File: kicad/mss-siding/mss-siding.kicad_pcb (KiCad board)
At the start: 2 copper layers, 82.6 x 76.2 mm, 108 parts, among them J1 Screw_Terminal_01x02, J10 Screw_Terminal_01x02, J11 Molex 0532610471, J12 Molex 0532610471, J2 SM04B-SRSS, J3 SM04B-SRSS, J4 SM04B-SRSS, J5 8P8C, J6 8P8C, J7 AVR-ISP, J8 Screw_Terminal_01x02, J9 Screw_Terminal_01x02, SW1 JS202011SCQN, U1 AP7381-50Y, U2 ATtiny861A-S, U3 74HC4049, U4 AP3012

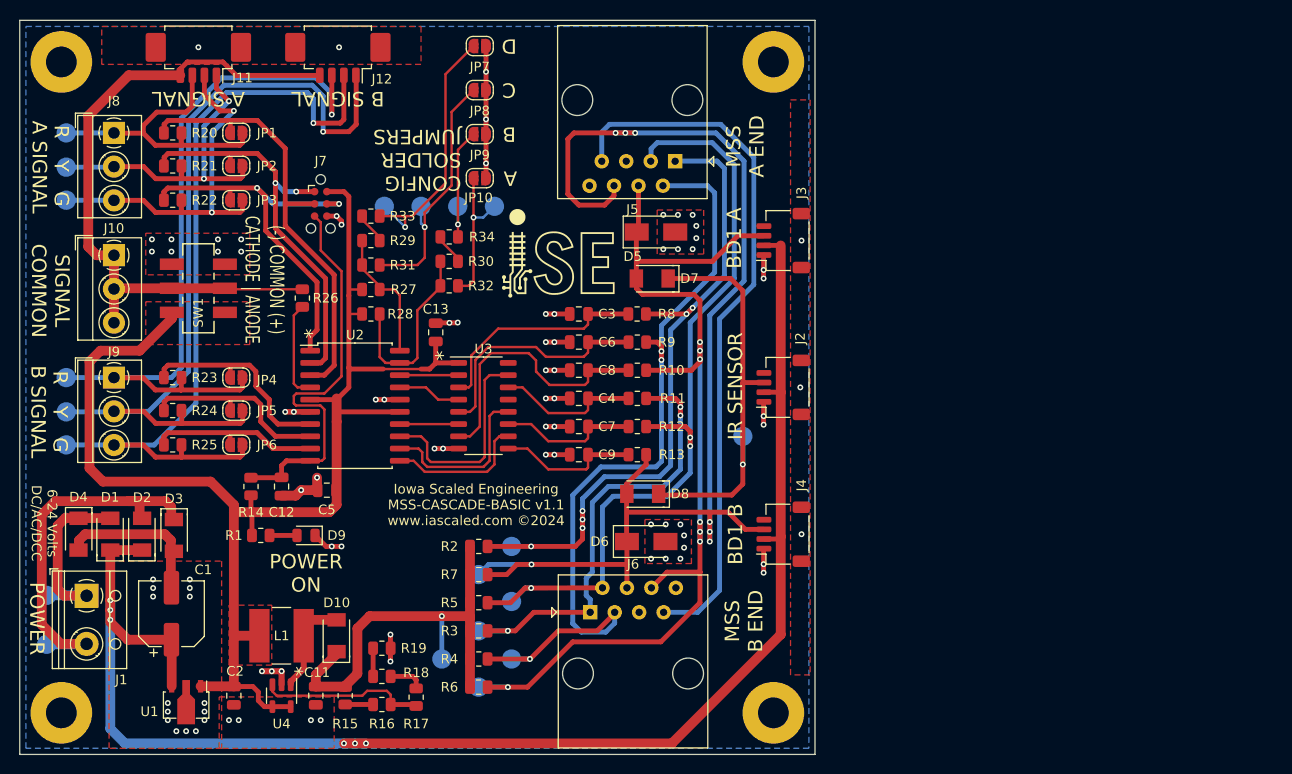
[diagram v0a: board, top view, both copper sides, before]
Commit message: First cut of PCB
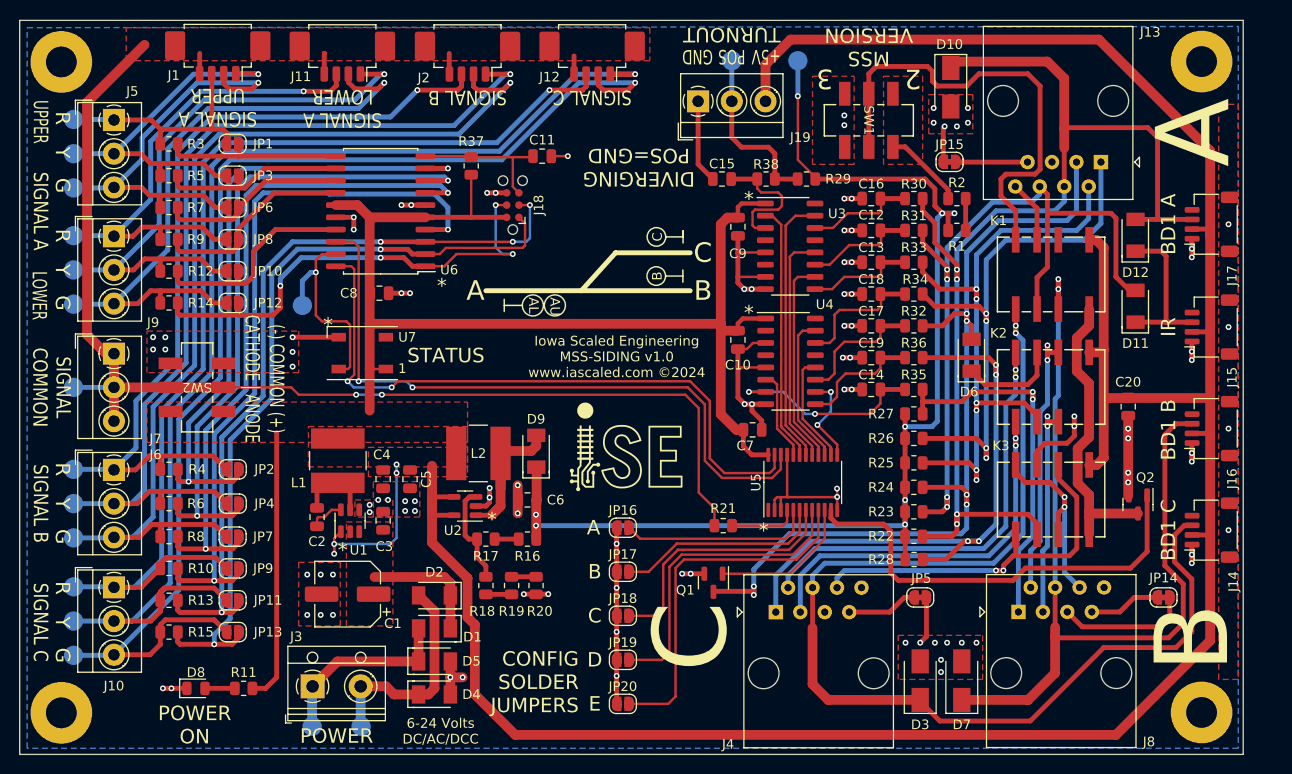
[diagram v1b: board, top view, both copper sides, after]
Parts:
- removed TP19, TP20: TestPoint, TestPoint:TestPoint_Pad_D2.0mm
- added C10: 0.1uF, Capacitor_SMD:C_0805_2012Metric, F.Cu at (99.9, 148.7)
- added C14: 0.1uF, Capacitor_SMD:C_0805_2012Metric, F.Cu at (113.8, 153.9)
- added C15: 0.1uF, Capacitor_SMD:C_0805_2012Metric, F.Cu at (98.3, 132.0)
- added C16: 0.1uF, Capacitor_SMD:C_0805_2012Metric, F.Cu at (113.8, 134.1)
- added C17: 0.1uF, Capacitor_SMD:C_0805_2012Metric, F.Cu at (113.8, 147.3)
- added C18: 0.1uF, Capacitor_SMD:C_0805_2012Metric, F.Cu at (113.8, 144.0)
- added C19: 0.1uF, Capacitor_SMD:C_0805_2012Metric, F.Cu at (113.8, 150.6)
- added C20: 10uF, Capacitor_SMD:C_0805_2012Metric, F.Cu at (140.5, 155.7)
- added D11: CDBM140G, ISE_Generic:SOD-123T, F.Cu at (141.2, 145.2)
- added D12: CDBM140G, ISE_Generic:SOD-123T, F.Cu at (141.2, 137.9)
- added J13: 8P8C, Connector_RJ:RJ45_Amphenol_54602-x08_Horizontal, F.Cu at (137.6, 130.3)
- added J14: SM04B-SRSS, Connector_JST:JST_SH_SM04B-SRSS-TB_1x04-1MP_P1.00mm_Horizontal, F.Cu at (149.1, 168.5)
- added J15: SM04B-SRSS, Connector_JST:JST_SH_SM04B-SRSS-TB_1x04-1MP_P1.00mm_Horizontal, F.Cu at (149.1, 147.4)
- added J16: SM04B-SRSS, Connector_JST:JST_SH_SM04B-SRSS-TB_1x04-1MP_P1.00mm_Horizontal, F.Cu at (149.1, 157.9)
- added J17: SM04B-SRSS, Connector_JST:JST_SH_SM04B-SRSS-TB_1x04-1MP_P1.00mm_Horizontal, F.Cu at (149.1, 136.7)
- added J18: AVR-ISP, Connector:Tag-Connect_TC2030-IDC-NL_2x03_P1.27mm_Vertical, F.Cu at (76.6, 134.7)
- added J19: Screw_Terminal_01x02, TerminalBlock_MetzConnect:TerminalBlock_MetzConnect_Type059_RT06303HBWC_1x03_P3.50mm_Horizontal, F.Cu at (95.8, 124.0)
- added JP11: SolderJumper_2_Open, Jumper:SolderJumper-2_P1.3mm_Open_RoundedPad1.0x1.5mm, F.Cu at (47.5, 175.8)
- added JP12: SolderJumper_2_Open, Jumper:SolderJumper-2_P1.3mm_Open_RoundedPad1.0x1.5mm, F.Cu at (47.5, 144.9)
- added JP13: SolderJumper_2_Open, Jumper:SolderJumper-2_P1.3mm_Open_RoundedPad1.0x1.5mm, F.Cu at (47.5, 179.1)
- added JP14: SolderJumper_2_Bridged, Jumper:SolderJumper-2_P1.3mm_Bridged_RoundedPad1.0x1.5mm, F.Cu at (144.1, 175.5)
- added JP15: SolderJumper_2_Bridged, Jumper:SolderJumper-2_P1.3mm_Bridged_RoundedPad1.0x1.5mm, F.Cu at (121.9, 130.3)
- added JP16: SolderJumper_2_Open, Jumper:SolderJumper-2_P1.3mm_Open_RoundedPad1.0x1.5mm, F.Cu at (88.0, 168.2)
- added JP17: SolderJumper_2_Open, Jumper:SolderJumper-2_P1.3mm_Open_RoundedPad1.0x1.5mm, F.Cu at (88.0, 172.8)
- added JP18: SolderJumper_2_Open, Jumper:SolderJumper-2_P1.3mm_Open_RoundedPad1.0x1.5mm, F.Cu at (88.0, 177.4)
- added JP19: SolderJumper_2_Open, Jumper:SolderJumper-2_P1.3mm_Open_RoundedPad1.0x1.5mm, F.Cu at (88.0, 182.0)
- added JP20: SolderJumper_2_Open, Jumper:SolderJumper-2_P1.3mm_Open_RoundedPad1.0x1.5mm, F.Cu at (88.0, 186.5)
- added K1: AGQ200A4H, ISE_UltraLibrarian:RELAY_AGQ_A_PAN, F.Cu at (132.5, 141.9)
- added K2: AGQ200A4H, ISE_UltraLibrarian:RELAY_AGQ_A_PAN, F.Cu at (132.5, 153.6)
- added K3: AGQ200A4H, ISE_UltraLibrarian:RELAY_AGQ_A_PAN, F.Cu at (132.5, 165.3)
- added L2: 4.7uH, ISE_UltraLibrarian:MSS6132-xxxMLC, F.Cu at (73.0, 160.5)
- added Q1: ZXMS6004FF, Package_TO_SOT_SMD:SOT-23, F.Cu at (97.4, 174.0)
- added Q2: DRDC3105-7, Package_TO_SOT_SMD:SOT-23, F.Cu at (141.5, 165.8)
- added R35: 10k, Resistor_SMD:R_0805_2012Metric, F.Cu at (118.2, 153.9)
- added R36: 10k, Resistor_SMD:R_0805_2012Metric, F.Cu at (118.2, 150.6)
- added R37: 10k, Resistor_SMD:R_0805_2012Metric, F.Cu at (72.3, 130.7)
- added R38: 10k, Resistor_SMD:R_0805_2012Metric, F.Cu at (102.9, 132.0)
- added SW2: JS202011SCQN, ISE_UltraLibrarian:SW_JS202011SCQN, F.Cu at (43.8, 153.7)
- added U5: PCA9555PW, Package_SO:TSSOP-24_4.4x7.8mm_P0.65mm, F.Cu at (106.7, 163.5)
- added U6: ATtiny861A-S, Package_SO:SOIC-20W_7.5x12.8mm_P1.27mm, F.Cu at (62.9, 135.4)
- added U7: WS2812B, LED_SMD:LED_WS2812B_PLCC4_5.0x5.0mm_P3.2mm, F.Cu at (61.0, 150.1)
- C11: value 10uF -> 1uF
- C12: value 1uF -> 0.1uF
- C2: value 22uF -> 0.1uF
- C3, C6: value 0.1uF -> 10uF
- C4, C5: value 0.1uF -> 22uF
- D10, D3, D7: value CDBM140G -> SMAJ18A-TP; footprint ISE_Generic:SOD-123T -> Diode_SMD:D_SMA
- D5, D6: value SMAJ18A-TP -> CDBM140G; footprint Diode_SMD:D_SMA -> ISE_Generic:SOD-123T
- D8: value CDBM140G -> GREEN LED; footprint ISE_Generic:SOD-123T -> LED_SMD:LED_0805_2012Metric
- D9: value GREEN LED -> CDBM140G; footprint LED_SMD:LED_0805_2012Metric -> ISE_Generic:SOD-123T
- J1: value Screw_Terminal_01x02 -> Molex 0532610471; footprint TerminalBlock_RND:TerminalBlock_RND_205-00012_1x02_P5.00mm_Horizontal -> Connector_Molex:Molex_PicoBlade_53261-0471_1x04-1MP_P1.25mm_Horizontal
- J2: value SM04B-SRSS -> Molex 0532610471; footprint Connector_JST:JST_SH_SM04B-SRSS-TB_1x04-1MP_P1.00mm_Horizontal -> Connector_Molex:Molex_PicoBlade_53261-0471_1x04-1MP_P1.25mm_Horizontal
- J3: value SM04B-SRSS -> Screw_Terminal_01x02; footprint Connector_JST:JST_SH_SM04B-SRSS-TB_1x04-1MP_P1.00mm_Horizontal -> TerminalBlock_RND:TerminalBlock_RND_205-00012_1x02_P5.00mm_Horizontal
- J4: value SM04B-SRSS -> 8P8C; footprint Connector_JST:JST_SH_SM04B-SRSS-TB_1x04-1MP_P1.00mm_Horizontal -> Connector_RJ:RJ45_Amphenol_54602-x08_Horizontal
- J5, J6: value 8P8C -> Screw_Terminal_01x02; footprint Connector_RJ:RJ45_Amphenol_54602-x08_Horizontal -> TerminalBlock_MetzConnect:TerminalBlock_MetzConnect_Type059_RT06303HBWC_1x03_P3.50mm_Horizontal
- J7: value AVR-ISP -> Screw_Terminal_01x02; footprint Connector:Tag-Connect_TC2030-IDC-NL_2x03_P1.27mm_Vertical -> TerminalBlock_MetzConnect:TerminalBlock_MetzConnect_Type059_RT06303HBWC_1x03_P3.50mm_Horizontal
- J8: value Screw_Terminal_01x02 -> 8P8C; footprint TerminalBlock_MetzConnect:TerminalBlock_MetzConnect_Type059_RT06303HBWC_1x03_P3.50mm_Horizontal -> Connector_RJ:RJ45_Amphenol_54602-x08_Horizontal
- JP5: value SolderJumper_2_Open -> SolderJumper_2_Bridged; footprint Jumper:SolderJumper-2_P1.3mm_Open_RoundedPad1.0x1.5mm -> Jumper:SolderJumper-2_P1.3mm_Bridged_RoundedPad1.0x1.5mm
- R10, R12, R13, R14, R15, R3, R4, R5, R6, R7, R8, R9: value 10k -> 330
- R11, R2: value 10k -> 1k
- R17: value 1k -> 10k
- R19: value 330 -> 1k
- R21, R22, R23, R24, R25: value 330 -> 10k
- U1: value AP7381-50Y -> AP63205WU; footprint ISE_Generic:SOT-89-3 -> Package_TO_SOT_SMD:TSOT-23-6
- U2: value ATtiny861A-S -> AP3012; footprint Package_SO:SOIC-20W_7.5x12.8mm_P1.27mm -> Package_TO_SOT_SMD:SOT-23-5
- U4: value AP3012 -> 74HC4049; footprint Package_TO_SOT_SMD:SOT-23-5 -> Package_SO:SO-16_3.9x9.9mm_P1.27mm
- moved J8 106.2 mm to (129.1, 177.0), turned to 0 degrees
- moved D10 85.5 mm to (122.0, 122.5), turned to -90 degrees
- moved R22 84.5 mm to (118.2, 169.1)
- moved H2 80.9 mm to (148.1, 119.8)
- moved H3 80.8 mm to (148.1, 187.4)
- moved D3 78.9 mm to (118.9, 184.1), turned to 90 degrees
- moved R1 78.9 mm to (122.7, 137.4)
- moved R23 78.2 mm to (118.2, 166.6)
- moved R24 77.4 mm to (118.2, 164.0)
- moved R25 77.0 mm to (118.2, 161.5), turned to 180 degrees
- moved JP5 73.6 mm to (118.9, 175.5), turned to 180 degrees
- moved SW1 71.7 mm to (113.5, 125.9), turned to -90 degrees
- moved TP2 68.8 mm to (60.8, 188.8)
- moved R21 68.3 mm to (98.4, 168.0), turned to 180 degrees
- moved J3 67.3 mm to (55.8, 184.7), turned to 0 degrees
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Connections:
- C1 pad 1: /VPWR -> Net-(C1-Pad1)
- C11 pad 1: +12V -> Net-(C11-Pad1)
- C13 pad 1: +5V -> Net-(C13-Pad1)
- C2 pad 1: +5V -> Net-(C2-Pad1)
- C2 pad 2: GND -> Net-(C2-Pad2)
- C3 pad 1: Net-(C3-Pad1) -> Net-(C1-Pad1)
- C4 pad 1: Net-(C4-Pad1) -> +5V
- C6 pad 1: Net-(C6-Pad1) -> +12V
- C7 pad 1: Net-(C7-Pad1) -> +5V
- C8 pad 1: Net-(C8-Pad1) -> +5V
- C9 pad 1: Net-(C9-Pad1) -> +5V
- D1 pad 1: /VPWR -> Net-(C1-Pad1)
- D10 pad 1: +12V -> /POINTS_S
- D10 pad 2: Net-(D10-Pad2) -> GND
- D2 pad 1: /VPWR -> Net-(C1-Pad1)
- D3 pad 1: Net-(D2-Pad2) -> /SIDE_S
- D4 pad 1: Net-(D1-Pad2) -> Net-(D2-Pad2)
- D5 pad 1: /A_ADJACENT -> Net-(D1-Pad2)
- D6 pad 1: /B_ADJACENT -> Net-(D6-Pad1)
- D6 pad 2: GND -> /POINTS_AA_OUT
- D7 pad 1: Net-(D7-Pad1) -> /MAIN_S
- D7 pad 2: /A_ADJACENT -> GND
- D8 pad 1: Net-(D7-Pad1) -> GND
- D8 pad 2: /B_ADJACENT -> Net-(D8-Pad2)
- D9 pad 1: GND -> +12V
- J1 pad 1: Net-(D1-Pad2) -> Net-(J1-Pad1)
- J1 pad 2: Net-(D2-Pad2) -> Net-(J1-Pad2)
- J10 pad 2: Net-(J10-Pad1) -> Net-(J10-Pad2)
- J10 pad 3: Net-(J10-Pad1) -> Net-(J10-Pad3)
- J11 pad 1: Net-(J8-Pad2) -> Net-(J11-Pad1)
- J11 pad 2: Net-(JP3-Pad2) -> Net-(J11-Pad2)
- J11 pad 3: Net-(J8-Pad1) -> Net-(J9-Pad1)
- J11 pad 4: Net-(J10-Pad1) -> Net-(J1-Pad4)
- J11 pad MP: GND -> Net-(J1-Pad4)
- J12 pad 1: Net-(J9-Pad2) -> Net-(J10-Pad2)
- J12 pad 2: Net-(JP6-Pad2) -> Net-(J10-Pad3)
- J12 pad 3: Net-(JP4-Pad2) -> Net-(J10-Pad1)
- J12 pad 4: Net-(J10-Pad1) -> Net-(J1-Pad4)
- J12 pad MP: GND -> Net-(J1-Pad4)
- J2 pad 1: GND -> Net-(J2-Pad1)
- J2 pad 2: /VPWR -> Net-(J2-Pad2)
- J2 pad 3: Net-(D7-Pad1) -> Net-(J2-Pad3)
- J2 pad 4: unconnected-(J2-Pad4) -> Net-(J1-Pad4)
- J2 pad MP: GND -> Net-(J1-Pad4)
- J3 pad 1: GND -> Net-(D1-Pad2)
- J3 pad 2: /VPWR -> Net-(D2-Pad2)
- J4 pad 1: GND -> /SIDE_AA_IN
- J4 pad 2: /VPWR -> /SIDE_A_IN
- J4 pad 3: /B_ADJACENT -> /SIDE_AA_OUT
- J4 pad 4: unconnected-(J4-Pad4) -> /SIDE_S
- J5 pad 1: Net-(J5-Pad1) -> Net-(J1-Pad3)
- J5 pad 2: Net-(J5-Pad2) -> Net-(J1-Pad1)
- J5 pad 3: Net-(J5-Pad3) -> Net-(J1-Pad2)
- J6 pad 1: Net-(J6-Pad1) -> Net-(J2-Pad3)
- J6 pad 2: Net-(J5-Pad3) -> Net-(J2-Pad1)
- J6 pad 3: Net-(J5-Pad2) -> Net-(J2-Pad2)
- J7 pad 1: /A_SIGNAL_Y -> Net-(J1-Pad4)
- J7 pad 2: +5V -> Net-(J1-Pad4)
- J7 pad 3: /A_SIGNAL_R -> Net-(J1-Pad4)
- J8 pad 1: Net-(J8-Pad1) -> /MAIN_AA_IN
- J8 pad 2: Net-(J8-Pad2) -> /MAIN_A_IN
- J8 pad 3: Net-(JP3-Pad2) -> /MAIN_AA_OUT
- J9 pad 1: Net-(JP4-Pad2) -> Net-(J9-Pad1)
- J9 pad 2: Net-(J9-Pad2) -> Net-(J11-Pad1)
- J9 pad 3: Net-(JP6-Pad2) -> Net-(J11-Pad2)
- JP1 pad 1: /A_SIGNAL_R -> /A_U_SIGNAL_R
- JP1 pad 2: Net-(J8-Pad1) -> Net-(J1-Pad3)
- JP10 pad 1: Net-(JP10-Pad1) -> /A_L_SIGNAL_Y
- JP10 pad 2: GND -> Net-(J11-Pad1)
- JP2 pad 1: /A_SIGNAL_Y -> /B_SIGNAL_R
- JP2 pad 2: Net-(J8-Pad2) -> Net-(J2-Pad3)
- JP3 pad 1: /A_SIGNAL_G -> /A_U_SIGNAL_Y
- JP3 pad 2: Net-(JP3-Pad2) -> Net-(J1-Pad1)
- JP4 pad 1: /B_SIGNAL_R -> /B_SIGNAL_Y
- JP4 pad 2: Net-(JP4-Pad2) -> Net-(J2-Pad1)
- JP5 pad 1: /B_SIGNAL_Y -> GND
- JP5 pad 2: Net-(J9-Pad2) -> Net-(J4-Pad7)
- JP6 pad 1: /B_SIGNAL_G -> /A_U_SIGNAL_G
- JP6 pad 2: Net-(JP6-Pad2) -> Net-(J1-Pad2)
- JP7 pad 1: Net-(TP19-Pad1) -> /B_SIGNAL_G
- JP7 pad 2: GND -> Net-(J2-Pad2)
- JP8 pad 1: Net-(JP8-Pad1) -> /A_L_SIGNAL_R
- JP8 pad 2: GND -> Net-(J9-Pad1)
- JP9 pad 1: Net-(JP9-Pad1) -> /C_SIGNAL_R
- JP9 pad 2: GND -> Net-(J10-Pad1)
- L1 pad 2: Net-(D10-Pad2) -> Net-(C2-Pad1)
- R1 pad 1: Net-(D9-Pad2) -> Net-(R1-Pad1)
- R1 pad 2: +5V -> +12V
- R10 pad 1: Net-(C8-Pad1) -> /C_SIGNAL_R
- R10 pad 2: /A_ADJACENT -> Net-(J10-Pad1)
- R11 pad 1: Net-(C4-Pad1) -> Net-(D8-Pad2)
- R11 pad 2: Net-(J6-Pad1) -> +5V
- R12 pad 1: Net-(C7-Pad1) -> /A_L_SIGNAL_Y
- R12 pad 2: Net-(J5-Pad3) -> Net-(J11-Pad1)
- R13 pad 1: Net-(C9-Pad1) -> /C_SIGNAL_Y
- R13 pad 2: /B_ADJACENT -> Net-(J10-Pad2)
- R14 pad 1: Net-(C12-Pad1) -> /A_L_SIGNAL_G
- R14 pad 2: +5V -> Net-(J11-Pad2)
- R15 pad 1: Net-(R15-Pad1) -> /C_SIGNAL_G
- R15 pad 2: +12V -> Net-(J10-Pad3)
- R16 pad 2: Net-(R15-Pad1) -> +12V
- R19 pad 1: GND -> Net-(R19-Pad1)
- R2 pad 1: Net-(J5-Pad1) -> Net-(R2-Pad1)
- R2 pad 2: +12V -> Net-(R1-Pad1)
- R20 pad 1: /A_SIGNAL_R -> GND
- R20 pad 2: Net-(J8-Pad1) -> Net-(R19-Pad1)
- R21 pad 1: /A_SIGNAL_Y -> /COM_SENSE
- R21 pad 2: Net-(J8-Pad2) -> Net-(J1-Pad4)
- R22 pad 1: /A_SIGNAL_G -> +12V
- R22 pad 2: Net-(JP3-Pad2) -> /POINTS_S
- R23 pad 1: /B_SIGNAL_R -> +12V
- R23 pad 2: Net-(JP4-Pad2) -> /POINTS_A_OUT
- R24 pad 1: /B_SIGNAL_Y -> +12V
- R24 pad 2: Net-(J9-Pad2) -> /POINTS_AA_OUT
- R25 pad 1: /B_SIGNAL_G -> /POINTS_A_IN
- R25 pad 2: Net-(JP6-Pad2) -> +12V
- R26 pad 1: Net-(J10-Pad1) -> +12V
- R26 pad 2: /COM_SENSE -> /POINTS_AA_IN
- R27 pad 1: /OPTIONS_1 -> +12V
- R27 pad 2: +5V -> /MAIN_AA_IN
- R28 pad 1: /OPTIONS_2 -> +12V
- R28 pad 2: +5V -> /SIDE_AA_IN
- R29 pad 1: Net-(R29-Pad1) -> +12V
- R29 pad 2: /OPTIONS_1 -> /TO_NORMAL
- R3 pad 1: Net-(J6-Pad1) -> /A_U_SIGNAL_R
- R3 pad 2: +12V -> Net-(J1-Pad3)
- R30 pad 1: Net-(R30-Pad1) -> /POINTS_S
- R30 pad 2: /OPTIONS_2 -> Net-(C16-Pad1)
- R31 pad 1: Net-(JP8-Pad1) -> /POINTS_A_OUT
- R31 pad 2: /OPTIONS_1 -> Net-(C12-Pad1)
- R32 pad 1: Net-(JP10-Pad1) -> /POINTS_AA_OUT
- R32 pad 2: /OPTIONS_2 -> Net-(C17-Pad1)
- R33 pad 1: Net-(TP19-Pad1) -> /POINTS_A_IN
- R33 pad 2: Net-(R29-Pad1) -> Net-(C13-Pad1)
- R34 pad 1: Net-(JP9-Pad1) -> /POINTS_AA_IN
- R34 pad 2: Net-(R30-Pad1) -> Net-(C18-Pad1)
- R4 pad 1: Net-(J5-Pad2) -> /B_SIGNAL_R
- R4 pad 2: +12V -> Net-(J2-Pad3)
- R5 pad 1: Net-(J5-Pad3) -> /A_U_SIGNAL_Y
- R5 pad 2: +12V -> Net-(J1-Pad1)
- R6 pad 1: /A_ADJACENT -> /B_SIGNAL_Y
- R6 pad 2: +12V -> Net-(J2-Pad1)
- R7 pad 1: /B_ADJACENT -> /A_U_SIGNAL_G
- R7 pad 2: +12V -> Net-(J1-Pad2)
- R8 pad 1: Net-(C3-Pad1) -> /B_SIGNAL_G
- R8 pad 2: Net-(J5-Pad1) -> Net-(J2-Pad2)
- R9 pad 1: Net-(C6-Pad1) -> /A_L_SIGNAL_R
- R9 pad 2: Net-(J5-Pad2) -> Net-(J9-Pad1)
- SW1 pad 1: +5V -> Net-(R2-Pad1)
- SW1 pad 2: Net-(J10-Pad1) -> Net-(K1-Pad4)
- SW1 pad 4: +5V -> Net-(R2-Pad1)
- SW1 pad 5: Net-(J10-Pad1) -> Net-(K1-Pad4)
- TP1 pad 1: Net-(D7-Pad1) -> Net-(D1-Pad2)
- TP10 pad 1: Net-(J6-Pad1) -> Net-(J10-Pad1)
- TP11 pad 1: Net-(J5-Pad1) -> Net-(J11-Pad1)
- TP12 pad 1: Net-(J5-Pad2) -> Net-(J10-Pad2)
- TP13 pad 1: /A_ADJACENT -> Net-(J11-Pad2)
- TP14 pad 1: /B_ADJACENT -> Net-(J10-Pad3)
- TP15 pad 1: Net-(J5-Pad3) -> +12V
- TP16 pad 1: +12V -> Net-(J1-Pad4)
- TP17 pad 1: Net-(JP8-Pad1) -> Net-(TP17-Pad1)
- TP18 pad 1: Net-(JP10-Pad1) -> /TO_NORMAL
- TP2 pad 1: Net-(J8-Pad1) -> Net-(D2-Pad2)
- TP3 pad 1: Net-(J8-Pad2) -> Net-(J1-Pad3)
- TP4 pad 1: Net-(JP3-Pad2) -> Net-(J2-Pad3)
- TP5 pad 1: Net-(JP4-Pad2) -> Net-(J1-Pad1)
- TP6 pad 1: Net-(J9-Pad2) -> Net-(J2-Pad1)
- TP7 pad 1: Net-(JP6-Pad2) -> Net-(J1-Pad2)
- TP8 pad 1: Net-(D1-Pad2) -> Net-(J2-Pad2)
- TP9 pad 1: Net-(D2-Pad2) -> Net-(J9-Pad1)
- U1 pad 2: GND -> Net-(C1-Pad1)
- U1 pad 3: /VPWR -> Net-(C1-Pad1)
- U2 pad 1: /A_SIGNAL_G -> Net-(D9-Pad2)
- U2 pad 2: /A_SIGNAL_Y -> GND
- U2 pad 3: /A_SIGNAL_R -> Net-(R17-Pad1)
- U2 pad 4: /COM_SENSE -> +5V
- U3 pad 10: /B_ADJACENT_5V -> Net-(U5-Pad16)
- U3 pad 11: Net-(C7-Pad1) -> Net-(C12-Pad1)
- U3 pad 12: /B_APPROACH_5V -> Net-(U5-Pad17)
- U3 pad 14: Net-(C4-Pad1) -> Net-(C16-Pad1)
- U3 pad 15: /B_ADV_APPROACH_5V -> Net-(U3-Pad15)
- U3 pad 2: /A_ADV_APPROACH_5V -> Net-(U3-Pad2)
- U3 pad 3: Net-(C3-Pad1) -> Net-(R38-Pad2)
- U3 pad 4: /A_APPROACH_5V -> unconnected-(U3-Pad4)
- U3 pad 5: Net-(C6-Pad1) -> GND
- U3 pad 6: /A_ADJACENT_5V -> unconnected-(U3-Pad6)
- U3 pad 7: Net-(C8-Pad1) -> GND
- U3 pad 9: Net-(C9-Pad1) -> Net-(C13-Pad1)
- U4 pad 1: Net-(D10-Pad2) -> +5V
- U4 pad 2: GND -> unconnected-(U4-Pad2)
- U4 pad 3: Net-(R16-Pad1) -> GND
- U4 pad 4: +5V -> unconnected-(U4-Pad4)
- U4 pad 5: +5V -> GND
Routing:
- net +5V: track 149.2 -> 434.0 mm, vias 0 -> 4
- net /VPWR: track 158.5 -> 0.00 mm, vias 6 -> 0
- net Net-(J1-Pad4): track 0.00 -> 130.0 mm, vias 0 -> 2
- net /B_ADJACENT: track 128.6 -> 0.00 mm, vias 7 -> 0
- net Net-(J10-Pad3): track 0.00 -> 126.4 mm, vias 0 -> 1
- net Net-(J10-Pad2): track 0.00 -> 122.1 mm, vias 0 -> 1
- net /POINTS_S: track 0.00 -> 118.6 mm, vias 0 -> 4
- net /SIDE_S: track 0.00 -> 117.2 mm, vias 0 -> 2
- net /A_ADJACENT: track 108.1 -> 0.00 mm, vias 7 -> 0
- net Net-(J2-Pad2): track 0.00 -> 103.8 mm, vias 0 -> 1
- net Net-(J2-Pad1): track 0.00 -> 98.2 mm, vias 0 -> 1
- net /POINTS_AA_OUT: track 0.00 -> 92.6 mm, vias 0 -> 6
- net /MAIN_S: track 0.00 -> 92.2 mm, vias 0 -> 2
- net Net-(J2-Pad3): track 0.00 -> 87.9 mm, vias 0 -> 1
- net GND: track 79.8 -> 166.7 mm, vias 88 -> 100
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- added copper zone on F.Cu, net Net-(C1-Pad1)
- added copper zone on F.Cu, net Net-(J1-Pad4)
- added copper zone on F.Cu, net Net-(R2-Pad1)
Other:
- board size 82.6 x 76.2 mm -> 127 x 76.2 mm
- board text added: "+5V"
- board text added: "2"
- board text added: "3"
- board text added: "AL"
- board text added: "AU"
- board text added: "BD1 C"
- board text added: "DIVERGING POS=GND"
- board text added: "E"
- board text added: "GND"
- board text added: "IR"
- board text added: "Iowa Scaled Engineering MSS-SIDING v1.0 www.iascaled.com ©2024"
- board text added: "LOWER"
- board text added: "MSS VERSION"
- board text added: "POS"
- board text added: "SIGNAL A"
- board text added: "SIGNAL A LOWER"
- board text added: "SIGNAL A UPPER"
- board text added: "SIGNAL B"
- board text added: "SIGNAL C"
- board text added: "STATUS"
- board text added: "TURNOUT"
- board text added: "UPPER"
- board text removed: "A SIGNAL"
- board text removed: "B SIGNAL"
- board text removed: "IR SENSOR"
- board text removed: "Iowa Scaled Engineering MSS-CASCADE-BASIC v1.1 www.iascaled.com ©2024"
- board text removed: "MSS A END"
- board text removed: "MSS B END"
